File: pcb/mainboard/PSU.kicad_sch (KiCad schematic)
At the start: 87 parts, among them J18 USB_C_Receptacle_USB2.0, J78 Conn_01x02_Pin, J83 Conn_01x02_Pin, Q5 2N7002, Q6 2N7002, Q7 NCE30P28Q, Q8 2N7002, SW2 SW_Push, U13 TL431DBZ, U14 CH224K, U15 SY8253ADC, U16 SY8253ADC

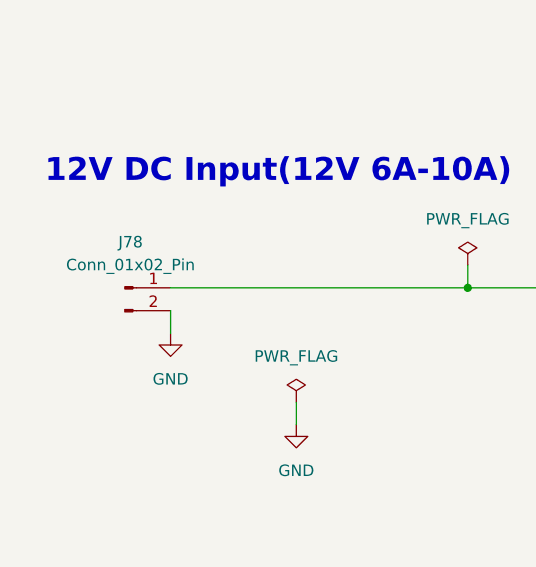
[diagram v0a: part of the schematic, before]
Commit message: before loading 12v in change
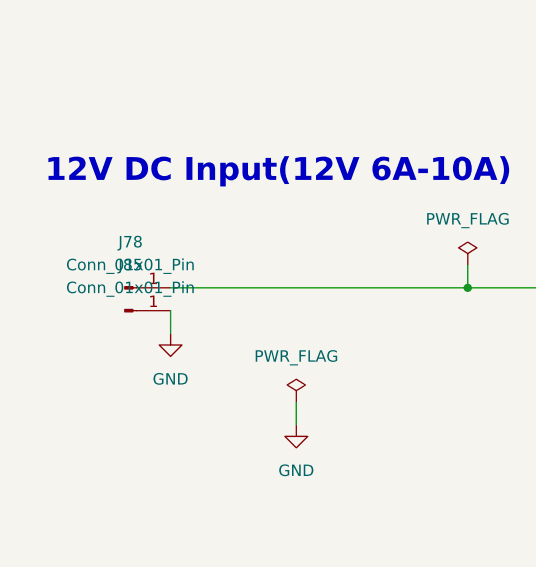
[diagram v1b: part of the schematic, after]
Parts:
- removed J78: Conn_01x02_Pin, Connector_PinHeader_2.54mm:PinHeader_1x02_P2.54mm_Vertical, symbol Connector:Conn_01x02_Pin
- added J78, J85: Conn_01x01_Pin, Connector_Wire:SolderWire-1sqmm_1x01_D1.4mm_OD2.7mm, symbol Connector:Conn_01x01_Pin
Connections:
- net +12V: now also J78.1 (Pin_1)
- net GND: now also J85.1 (Pin_1)
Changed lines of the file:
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@@
 	)
 	(symbol
-		(lib_id "Connector:Conn_01x02_Pin")
-		(at 171.45 163.83 0)
-		(unit 1)
-		(exclude_from_sim no)
-		(in_bom yes)
-		(on_board yes)
-		(dnp no)
-		(fields_autoplaced yes)
-		(property "Reference" "J78"
-			(at 172.085 158.75 0)
-			(effects
-				(font
-					(size 1.27 1.27)
-				)
-			)
-		)
-		(property "Value" "Conn_01x02_Pin"
-			(at 172.085 161.29 0)
-			(effects
-				(font
-					(size 1.27 1.27)
-				)
-			)
-		)
-		(property "Footprint" "Connector_PinHeader_2.54mm:PinHeader_1x02_P2.54mm_Vertical"
-			(at 171.45 163.83 0)
-			(effects
-				(font
-					(size 1.27 1.27)
-				)
-				(hide yes)
-			)
-		)
-		(property "Datasheet" "~"
-			(at 171.45 163.83 0)
-			(effects
-				(font
-					(size 1.27 1.27)
-				)
-				(hide yes)
-			)
-		)
-		(property "Description" "Generic connector, single row, 01x02, script generated"
-			(at 171.45 163.83 0)
-			(effects
-				(font
-					(size 1.27 1.27)
-				)
-				(hide yes)
-			)
-		)
-		(pin "1"
-		)
-		(pin "2"
-		)
-		(instances
-			(project ""
-				(path "/2a6d114a-7fd7-4207-b5f7-4ea9c34f36aa/b23aee49-27d1-466d-98e2-113ee657e42b"
-					(reference "J78")
-					(unit 1)
-				)
-			)
-		)
-	)
-	(symbol
 		(lib_id "Device:C")
 		(at 444.5 171.45 180)
@@
 	)
 	(symbol
+		(lib_id "Connector:Conn_01x01_Pin")
+		(at 171.45 166.37 0)
+		(unit 1)
+		(exclude_from_sim no)
+		(in_bom yes)
+		(on_board yes)
+		(dnp no)
+		(fields_autoplaced yes)
+		(property "Reference" "J85"
+			(at 172.085 161.29 0)
+			(effects
+				(font
+					(size 1.27 1.27)
+				)
+			)
+		)
+		(property "Value" "Conn_01x01_Pin"
+			(at 172.085 163.83 0)
+			(effects
+				(font
+					(size 1.27 1.27)
+				)
+			)
+		)
+		(property "Footprint" "Connector_Wire:SolderWire-1sqmm_1x01_D1.4mm_OD2.7mm"
+			(at 171.45 166.37 0)
+			(effects
+				(font
+					(size 1.27 1.27)
+				)
+				(hide yes)
+			)
+		)
+		(property "Datasheet" "~"
+			(at 171.45 166.37 0)
+			(effects
+				(font
+					(size 1.27 1.27)
+				)
+				(hide yes)
+			)
+		)
+		(property "Description" "Generic connector, single row, 01x01, script generated"
+			(at 171.45 166.37 0)
+			(effects
+				(font
+					(size 1.27 1.27)
+				)
+				(hide yes)
+			)
+		)
+		(pin "1"
+		)
+		(instances
+			(project "[DFR1142]Lite Carrier for LattePanda Mu"
+				(path "/2a6d114a-7fd7-4207-b5f7-4ea9c34f36aa/b23aee49-27d1-466d-98e2-113ee657e42b"
+					(reference "J85")
+					(unit 1)
+				)
+			)
+		)
+	)
+	(symbol
 		(lib_id "power:VDC")
 		(at 341.63 130.81 0)
@@
 					(unit 1)
 				)
+			)
+		)
+	)
+	(symbol
+		(lib_id "Connector:Conn_01x01_Pin")
+		(at 171.45 163.83 0)
+		(unit 1)
+		(exclude_from_sim no)
+		(in_bom yes)
+		(on_board yes)
+		(dnp no)
+		(fields_autoplaced yes)
+		(property "Reference" "J78"
+			(at 172.085 158.75 0)
+			(effects
+				(font
+					(size 1.27 1.27)
+				)
+			)
+		)
+		(property "Value" "Conn_01x01_Pin"
+			(at 172.085 161.29 0)
+			(effects
+				(font
+					(size 1.27 1.27)
+				)
+			)
+		)
+		(property "Footprint" "Connector_Wire:SolderWire-1sqmm_1x01_D1.4mm_OD2.7mm"
+			(at 171.45 163.83 0)
+			(effects
+				(font
+					(size 1.27 1.27)
+				)
+				(hide yes)
+			)
+		)
+		(property "Datasheet" "~"
+			(at 171.45 163.83 0)
+			(effects
+				(font
+					(size 1.27 1.27)
+				)
+				(hide yes)
+			)
+		)
+		(property "Description" "Generic connector, single row, 01x01, script generated"
+			(at 171.45 163.83 0)
+			(effects
+				(font
+					(size 1.27 1.27)
+				)
+				(hide yes)
+			)
+		)
+		(pin "1"
+		)
+		(instances
+			(project ""
+				(path "/2a6d114a-7fd7-4207-b5f7-4ea9c34f36aa/b23aee49-27d1-466d-98e2-113ee657e42b"
+					(reference "J78")
+					(unit 1)
+				)
